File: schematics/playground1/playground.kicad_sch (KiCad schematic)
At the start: 55 parts, among them SW1 SW_SPST, SW2 SW_Push, SW3 SW_Push, U1 ADS1299, U2 MCP1700x-330xxTT, U3 PIC32MX250F128B_I_SS, U5 LM2931AZ-5.0_TO92, Y1 8MHz

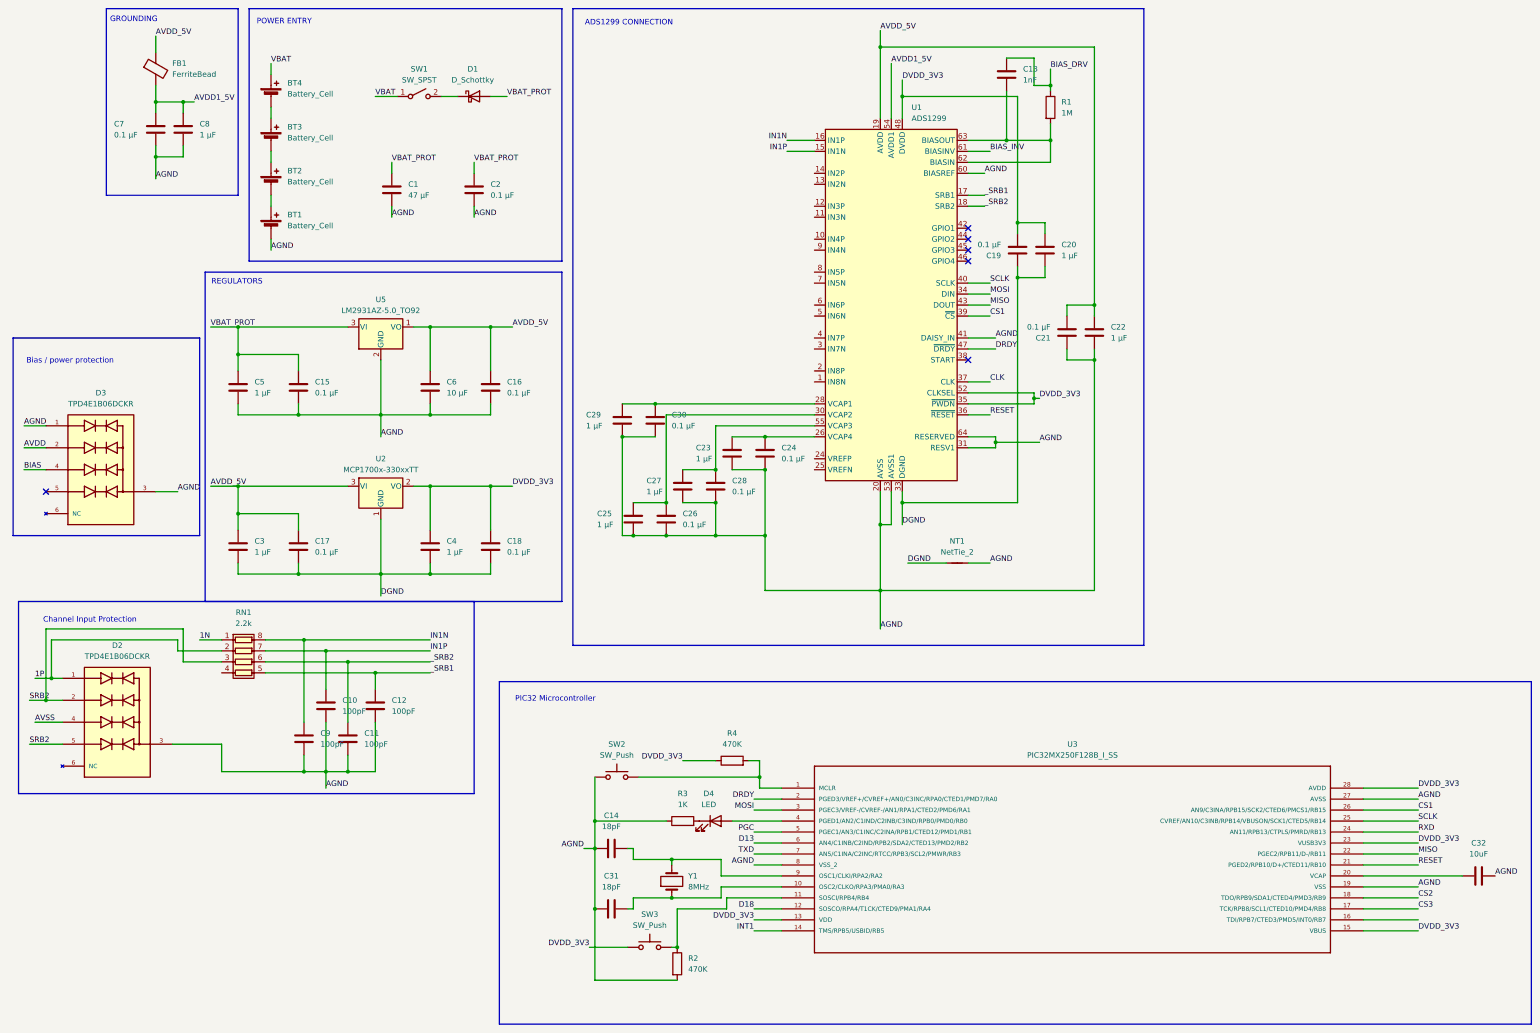
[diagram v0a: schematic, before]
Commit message: fix some errors
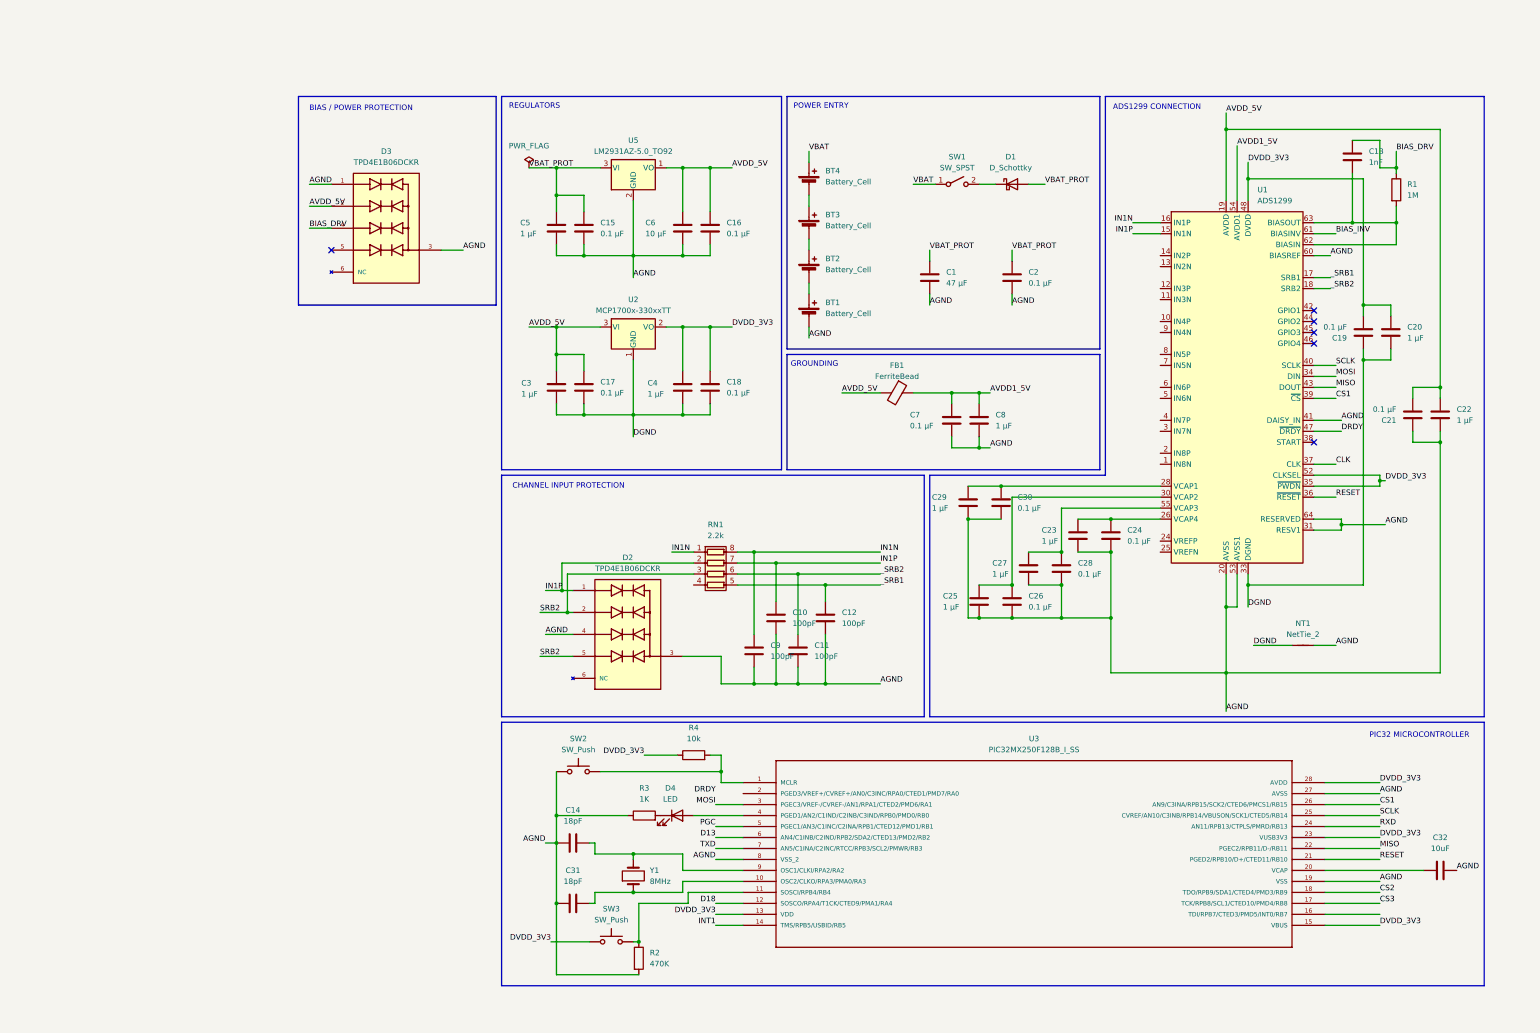
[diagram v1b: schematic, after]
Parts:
- C6: footprint (none) -> Capacitor_Tantalum_SMD:CP_EIA-3216-18_Kemet-A_HandSolder
- R4: value 470K -> 10k
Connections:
- net 1N is gone; now on net IN1N: RN1.1 (R1.1)
- net 1P is gone; now on net IN1P: D2.1, RN1.2 (R2.1)
- net AVDD is gone; now on net AVDD_5V: D3.2
- net AVSS is gone; now on net AGND: D2.4
- net BIAS is gone; now on net BIAS_DRV: D3.4
- net AGND: now also C6.1; no longer C6.2
- net AVDD1_5V: now also FB1.1; no longer FB1.2
- net AVDD_5V: now also C6.2, FB1.2; no longer C6.1, FB1.1
- net DRDY: no longer U3.2 (PGED3/VREF+/CVREF+/AN0/C3INC/RPA0/CTED1/PMD7/RA0)
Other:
- note added: "BIAS / POWER PROTECTION"
- note added: "CHANNEL INPUT PROTECTION"
- note added: "PIC32 MICROCONTROLLER"
- note removed: "Bias / power protection"
- note removed: "Channel Input Protection"
- note removed: "PIC32 Microcontroller"
- moved on the sheet: BT1, BT2, BT3, BT4, C1, C10, C11, C12, C13, C14, C15, C16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
